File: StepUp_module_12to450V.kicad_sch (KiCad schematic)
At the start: 0 parts

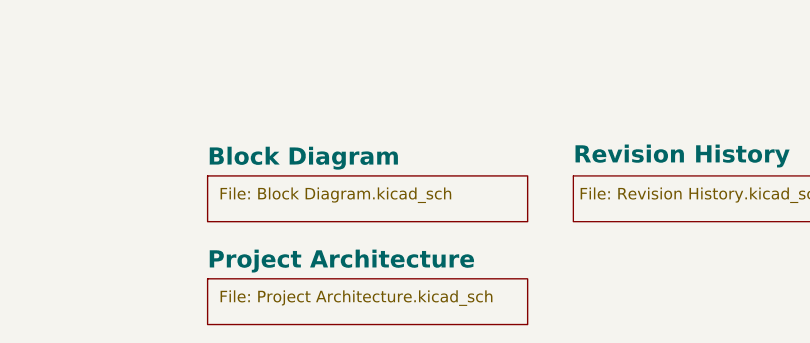
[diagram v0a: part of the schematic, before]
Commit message: testing lib issue
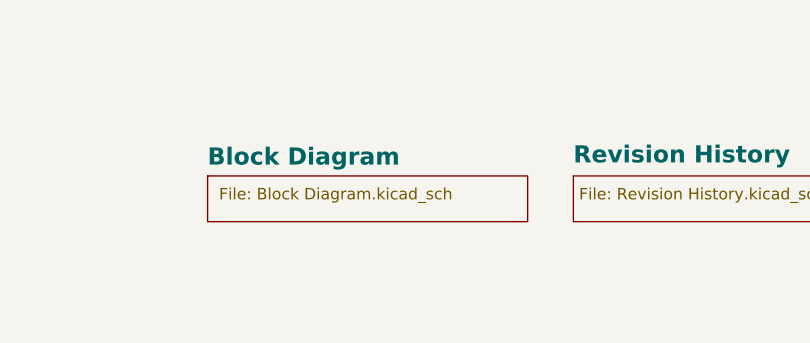
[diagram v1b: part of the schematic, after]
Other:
- removed sheet Project Architecture
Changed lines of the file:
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@@
 		(rev "${REVISION}")
 		(company "${COMPANY}")
+		(comment 9 "NA")
 	)
 	(text "Variant: ${VARIANT}"
@@
 			(project "StepUp_module_12to450V"
 				(path "/f9e05184-c88b-4a88-ae9c-ab2bdb32be7c"
-					(page "5")
+					(page "4")
 				)
 			)
@@
 				)
 			)
-		)
-	)
-	(sheet
-		(at 299.72 313.69)
-		(size 35.56 5.08)
-		(exclude_from_sim no)
-		(in_bom yes)
-		(on_board yes)
-		(dnp no)
-		(stroke
-			(width 0.1524)
-			(type solid)
-		)
-		(fill
-			(color 0 0 0 0.0000)
-		)
-		(property "Sheetname" "Project Architecture"
-			(at 299.72 312.6609 0)
-			(effects
-				(font
-					(face "Times New Roman")
-					(size 1.905 1.905)
-					(bold yes)
-					(color 0 0 0 1)
-				)
-				(justify left bottom)
-			)
-		)
-		(property "Sheetfile" "Project Architecture.kicad_sch"
-			(at 300.99 314.96 0)
-			(effects
-				(font
-					(face "Arial")
-					(size 1.27 1.27)
-				)
-				(justify left top)
-			)
-		)
-		(instances
-			(project "StepUp_module_12to450V"
-				(path "/f9e05184-c88b-4a88-ae9c-ab2bdb32be7c"
-					(page "3")
-				)
-			)

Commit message: DRC completed, changed status to checked
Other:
- note removed: "${SHEET_NAME_11}"
- note removed: "${SHEET_NAME_12}"
- note removed: "${SHEET_NAME_13}"
- note removed: "${SHEET_NAME_14}"
- note removed: "${SHEET_NAME_15}"
- note removed: "${SHEET_NAME_16}"
- note removed: "${SHEET_NAME_17}"
- note removed: "${SHEET_NAME_18}"
- note removed: "${SHEET_NAME_19}"
- note removed: "${SHEET_NAME_20}"
- note removed: "${SHEET_NAME_21}"
- note removed: "${SHEET_NAME_22}"
- note removed: "${SHEET_NAME_23}"
- note removed: "${SHEET_NAME_24}"
- note removed: "${SHEET_NAME_25}"
- note removed: "${SHEET_NAME_26}"
- note removed: "${SHEET_NAME_27}"
- note removed: "${SHEET_NAME_28}"
- note removed: "${SHEET_NAME_29}"
- note removed: "${SHEET_NAME_30}"
- note removed: "${SHEET_NAME_31}"
- note removed: "${SHEET_NAME_32}"
- note removed: "${SHEET_NAME_33}"
- note removed: "${SHEET_NAME_34}"
- note removed: "${SHEET_NAME_35}"
- note removed: "${SHEET_NAME_36}"
- note removed: "${SHEET_NAME_37}"
- note removed: "${SHEET_NAME_38}"
- note removed: "${SHEET_NAME_39}"
- note removed: "${SHEET_NAME_40}"
- note removed: "11"
- note removed: "12"
- note removed: "13"
- note removed: "14"
- note removed: "15"
- note removed: "16"
- note removed: "17"
- note removed: "18"
- note removed: "19"
- note removed: "20"
- note removed: "21"
- note removed: "22"
- note removed: "23"
- note removed: "24"
- note removed: "25"
- note removed: "26"
- note removed: "27"
- note removed: "28"
- note removed: "29"
- note removed: "30"
- note removed: "31"
- note removed: "32"
- note removed: "33"
- note removed: "34"
- note removed: "35"
- note removed: "36"
- note removed: "37"
- note removed: "38"
- note removed: "39"
- note removed: "40"

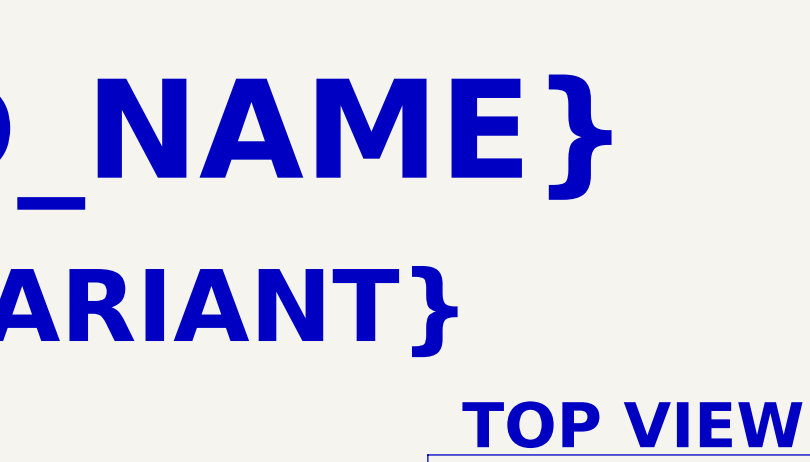
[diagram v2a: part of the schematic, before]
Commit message: Reverted?
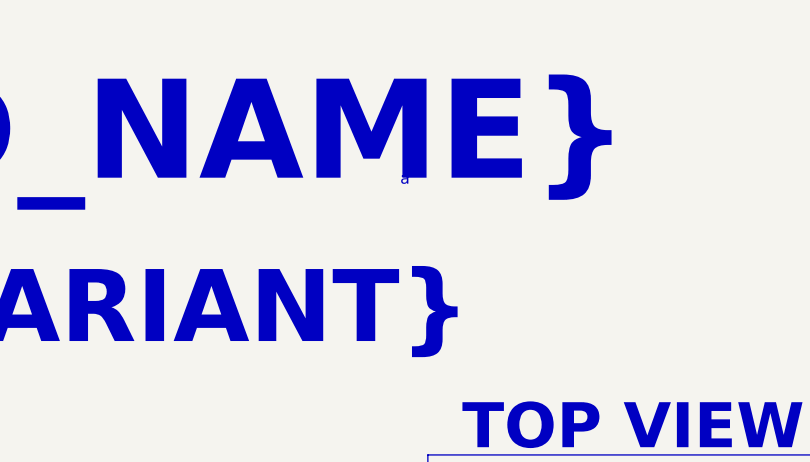
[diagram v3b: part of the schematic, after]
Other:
- note added: "a"
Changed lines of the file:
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@@
+		)
+	)
+	(text "a"
+		(exclude_from_sim no)
+		(at 149.86 39.37 0)
+		(effects
+			(font
+				(size 1.27 1.27)
+			)
 		)
 	)

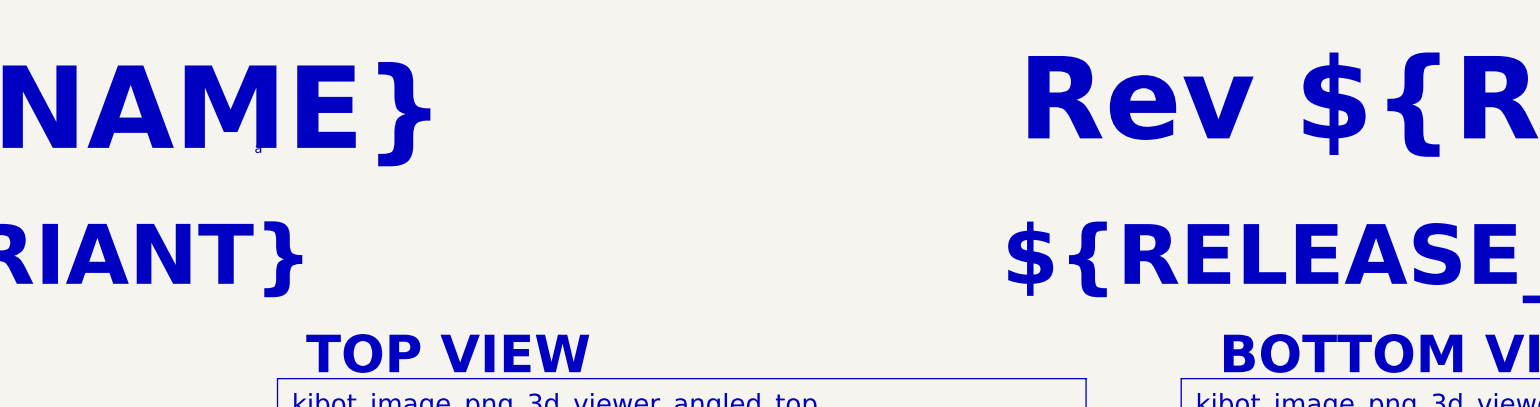
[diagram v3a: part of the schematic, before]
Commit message: DBG1
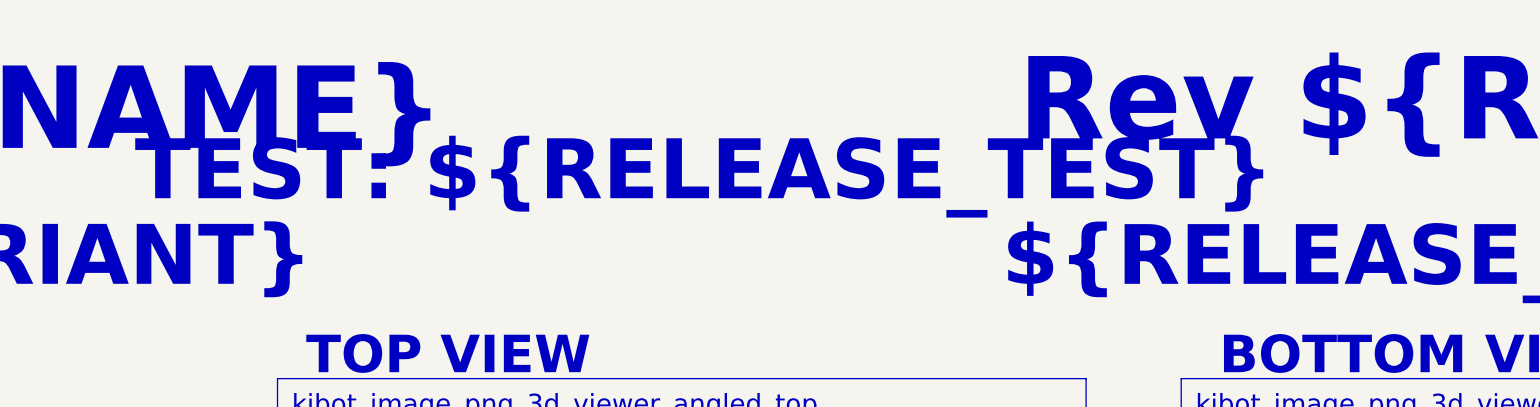
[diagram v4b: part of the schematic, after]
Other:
- note added: "TEST: ${RELEASE_TEST}"
- note removed: "a"
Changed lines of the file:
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@@
-		)
-	)
-	(text "a"
-		(exclude_from_sim no)
-		(at 149.86 39.37 0)
-		(effects
-			(font
-				(size 1.27 1.27)
-			)
 		)
 	)
@@
 			)
 			(justify left bottom)
+		)
+	)
+	(text "TEST: ${RELEASE_TEST}"
+		(exclude_from_sim no)
+		(at 133.35 46.99 0)
+		(effects
+			(font
+				(face "Times New Roman")
+				(size 8 8)
+				(thickness 1)
+				(bold yes)
+				(color 0 0 194 1)
+			)
+			(justify left bottom)

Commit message: DBG2
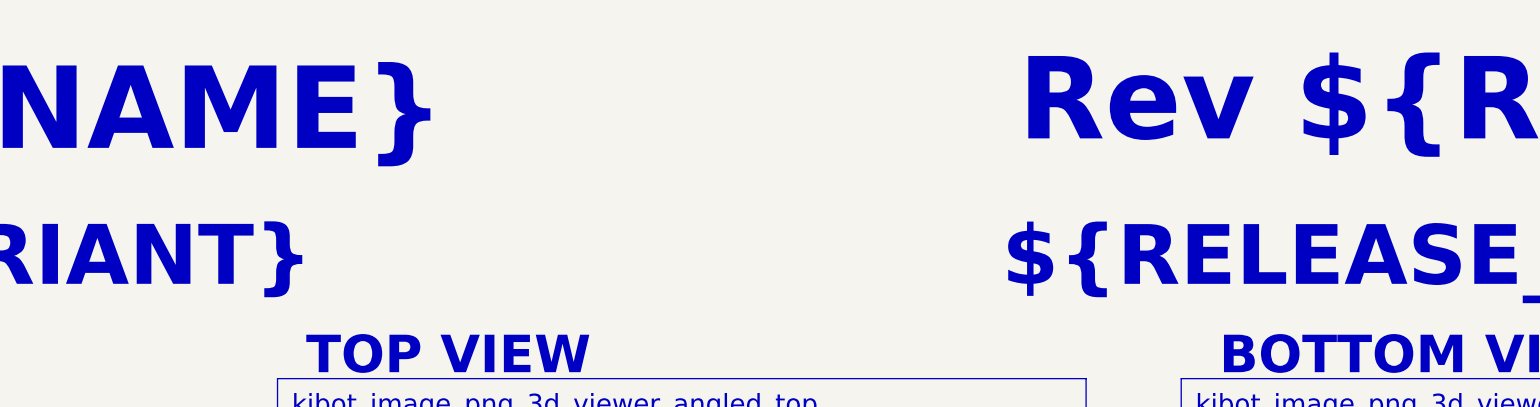
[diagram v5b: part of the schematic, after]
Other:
- note removed: "TEST: ${RELEASE_TEST}"
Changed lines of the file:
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@@
-		)
-	)
-	(text "TEST: ${RELEASE_TEST}"
-		(exclude_from_sim no)
-		(at 133.35 46.99 0)
-		(effects
-			(font
-				(face "Times New Roman")
-				(size 8 8)
-				(thickness 1)
-				(bold yes)
-				(color 0 0 194 1)
-			)
-			(justify left bottom)
 		)
 	)

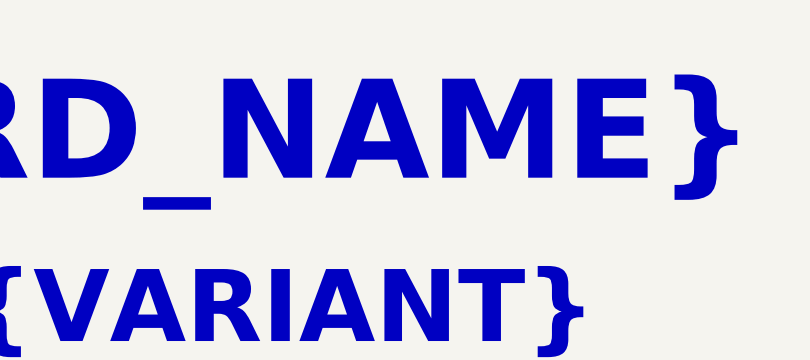
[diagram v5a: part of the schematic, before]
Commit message: DBG8
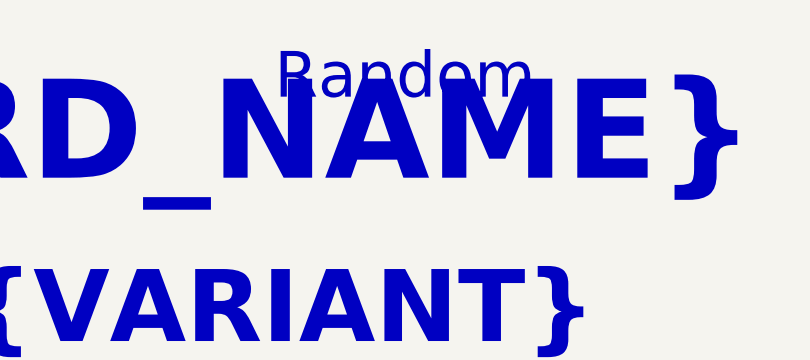
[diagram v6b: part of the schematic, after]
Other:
- note added: "Random"
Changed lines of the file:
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@@
+		)
+	)
+	(text "Random"
+		(exclude_from_sim no)
+		(at 135.89 27.94 0)
+		(effects
+			(font
+				(size 5.08 5.08)
+			)
 		)
 	)

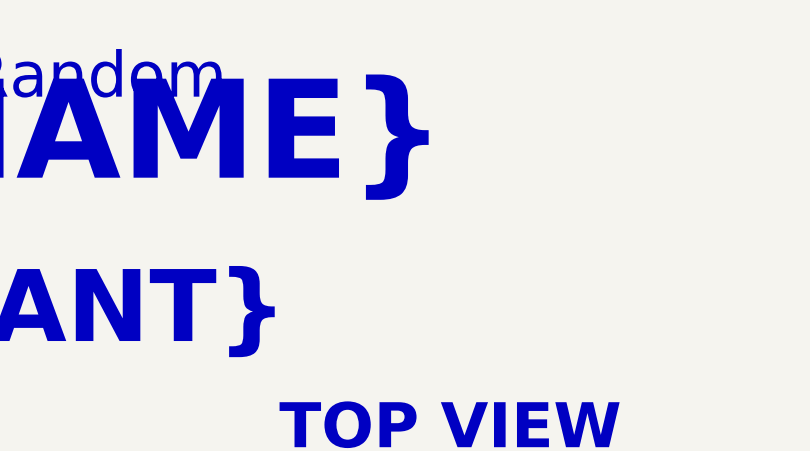
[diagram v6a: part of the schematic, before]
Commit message: DBG11
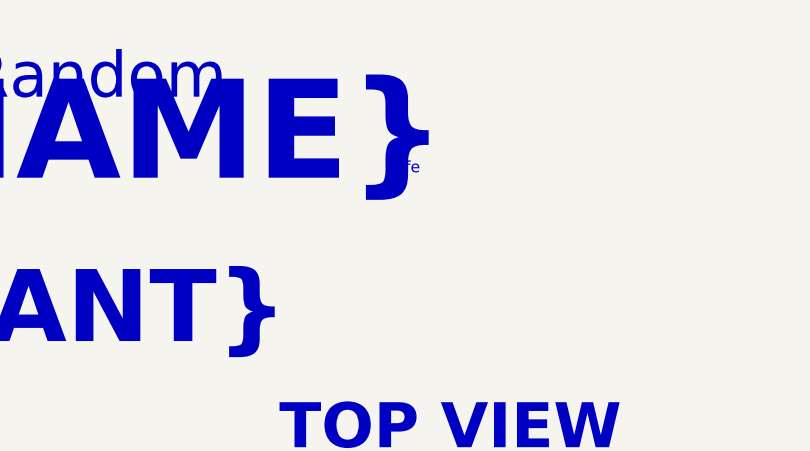
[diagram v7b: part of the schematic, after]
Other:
- note added: "fefe"
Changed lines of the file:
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@@
+		)
+	)
+	(text "fefe"
+		(exclude_from_sim no)
+		(at 170.18 38.1 0)
+		(effects
+			(font
+				(size 1.27 1.27)
+			)
 		)
 	)

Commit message: DBG11
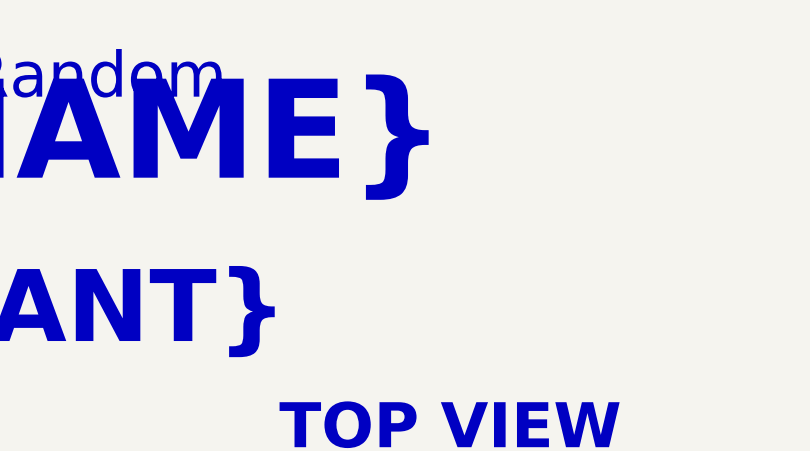
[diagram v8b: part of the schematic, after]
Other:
- note removed: "fefe"
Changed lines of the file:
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@@
-		)
-	)
-	(text "fefe"
-		(exclude_from_sim no)
-		(at 170.18 38.1 0)
-		(effects
-			(font
-				(size 1.27 1.27)
-			)
 		)
 	)
